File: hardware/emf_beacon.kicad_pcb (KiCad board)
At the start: 2 copper layers, 100 x 100 mm, 138 parts, among them J1 USB_C_Receptacle_USB2.0_16P, J10 Conn_01x02, J11 Conn_01x02, J12 Conn_01x02, J13 Conn_01x02, J14 Conn_01x02, J2 B6B-PH-SM4-TB, J3 B6B-PH-SM4-TB, J4 Conn_01x02, J5 Conn_01x02, J6 Conn_01x02, J7 Conn_01x02, J8 Conn_01x02, J9 Conn_01x02, Q1 AO3400A, Q10 AO3400A, Q11 AO3400A, Q12 DMP3013SFV, Q2 AO3400A, Q3 AO3400A, Q4 AO3400A, Q5 AO3400A, Q6 AO3400A, Q7 AO3400A, Q8 AO3400A, Q9 AO3400A, SW1 SW_DIP_x10, SW2 TS-1088-AR02016, U1 ESP32-C3-WROOM-02, U2 MCP23017T-E/SS, U4 PCA9685PW,118, U5 TPS565208, U6 CA-IS3092VW, U7 TPS82140SILR

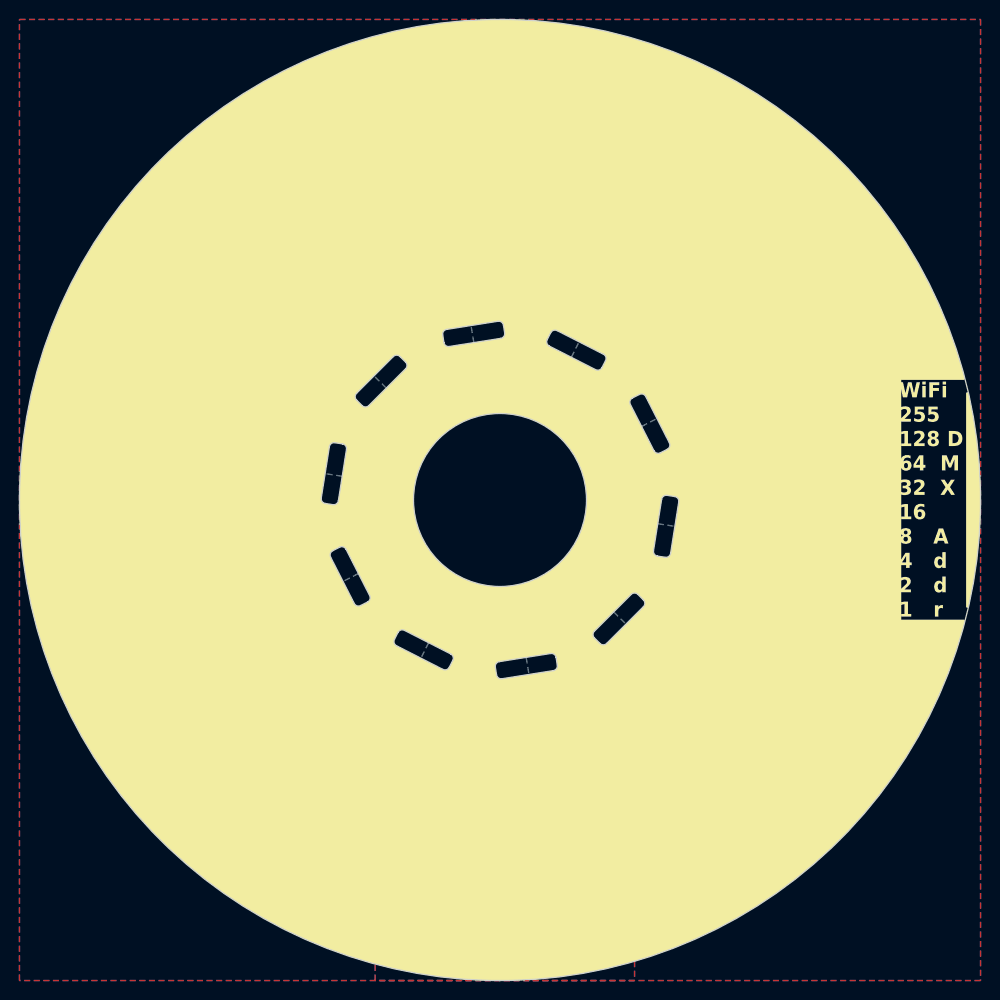
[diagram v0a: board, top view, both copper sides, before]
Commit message: more layout and fixing OOS items
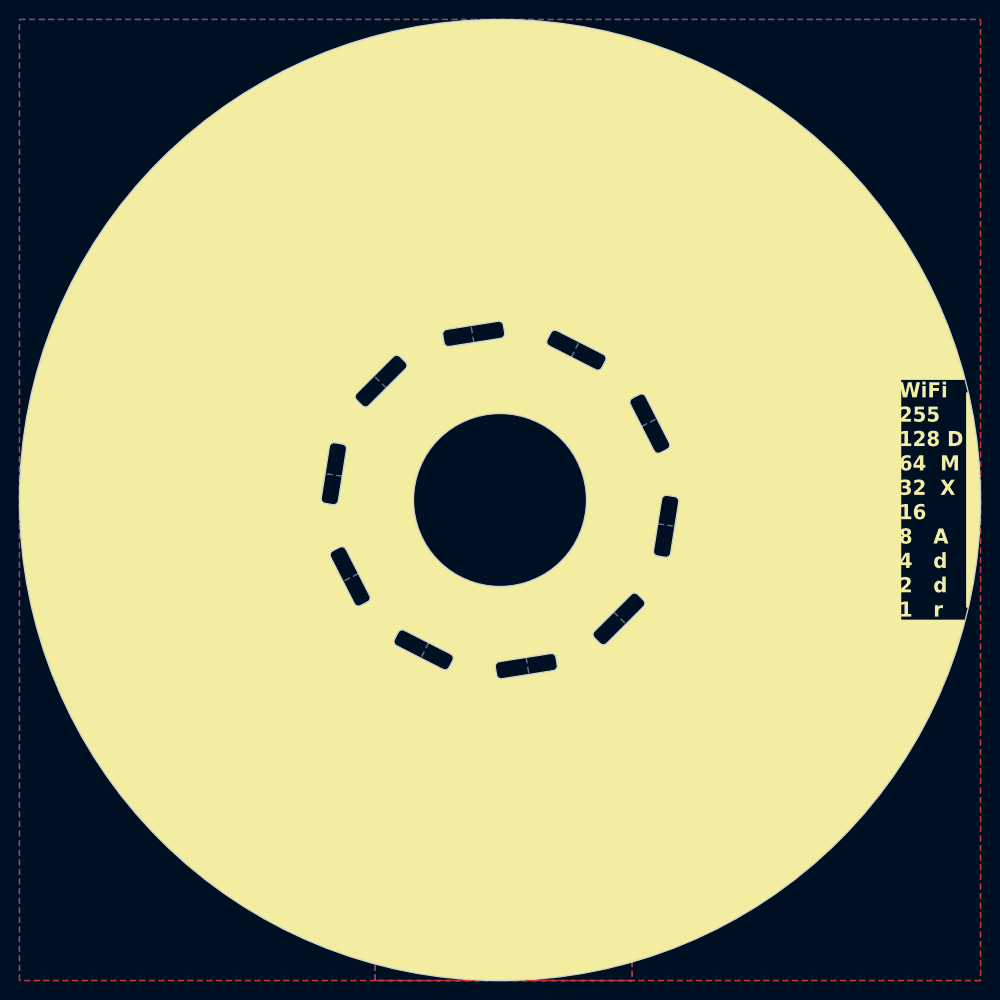
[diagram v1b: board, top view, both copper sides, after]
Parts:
- removed Q11: AO3400A, Package_TO_SOT_SMD:SOT-23
- removed R31: 100R, Resistor_SMD:R_0603_1608Metric
- removed R32, R33: 10k, Resistor_SMD:R_0603_1608Metric
- J10, J11, J12, J13, J4, J5, J6, J7, J8, J9: footprint Pinski1_parts:LED_Stick -> emf_beacon_library:LED_Stick
- J14: footprint TerminalBlock_WAGO:TerminalBlock_WAGO_2601-3102_1x02_P3.50mm_Vertical -> emf_beacon_library:MX250-3.5-02P-A-GY01-Cu-A
- L1: value MDE0840-3R3M -> MWSA0804S-3R3MT
- moved TP7 21.5 mm to (158.5, 121.2)
- moved C11 15.2 mm to (175.5, 85.5), turned to 0 degrees
- moved C9 9.65 mm to (172.8, 133.8)
- moved C10 9.58 mm to (174.5, 133.8)
- moved R15 8.22 mm to (170.2, 72.5)
- moved R11 7.00 mm to (157.2, 135.0)
- moved C16 2.30 mm to (172.0, 113.5), turned to -45 degrees
- moved R8 2.12 mm to (159.0, 146.2), turned to -90 degrees
- moved J14 1.83 mm to (129.8, 136.9), turned to 0 degrees
- moved C14 1.46 mm to (128.5, 128.8), turned to 180 degrees
- moved C5 1.41 mm to (156.5, 146.2), turned to -90 degrees
- moved C23 1.00 mm to (162.0, 131.0)
- moved C7 0.53 mm to (157.1, 132.8)
- moved C8 0.53 mm to (158.8, 133.0)
- moved R10 0.25 mm to (157.2, 140.0)
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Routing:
- net +3V3: track 177.6 -> 227.2 mm, vias 7 -> 11
- net /CTRL/DMX_DE/~{RE}: track 94.9 -> 113.0 mm
- net /CTRL/DMX_RX: track 79.3 -> 96.8 mm, vias 0 -> 2
- net /CTRL/DMX_TX: track 80.8 -> 96.9 mm
- net /DMX512/DMX_SHLD: track 9.00 -> 16.4 mm
- net /DMX512/DMX_DATA-: track 14.7 -> 19.6 mm
- net /DMX512/DMX_DATA+: track 14.7 -> 19.6 mm
- net +6V5: track 36.1 -> 40.8 mm
- net Net-(Q11-G): track 3.36 -> 0.00 mm
- net /LEDS/LED8: track 0.00 -> 2.09 mm
- net /LEDS/LED9: track 0.00 -> 2.05 mm
- net /CTRL/LED_~{PGD}: track 1.74 -> 0.00 mm
- net /I2C_SDA: track 51.1 -> 52.5 mm
- net /I2C_SCL: track 49.1 -> 50.6 mm
- net GND_ISO: vias 2 -> 15
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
